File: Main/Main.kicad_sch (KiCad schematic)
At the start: 2 parts, among them J1 ATMEGA

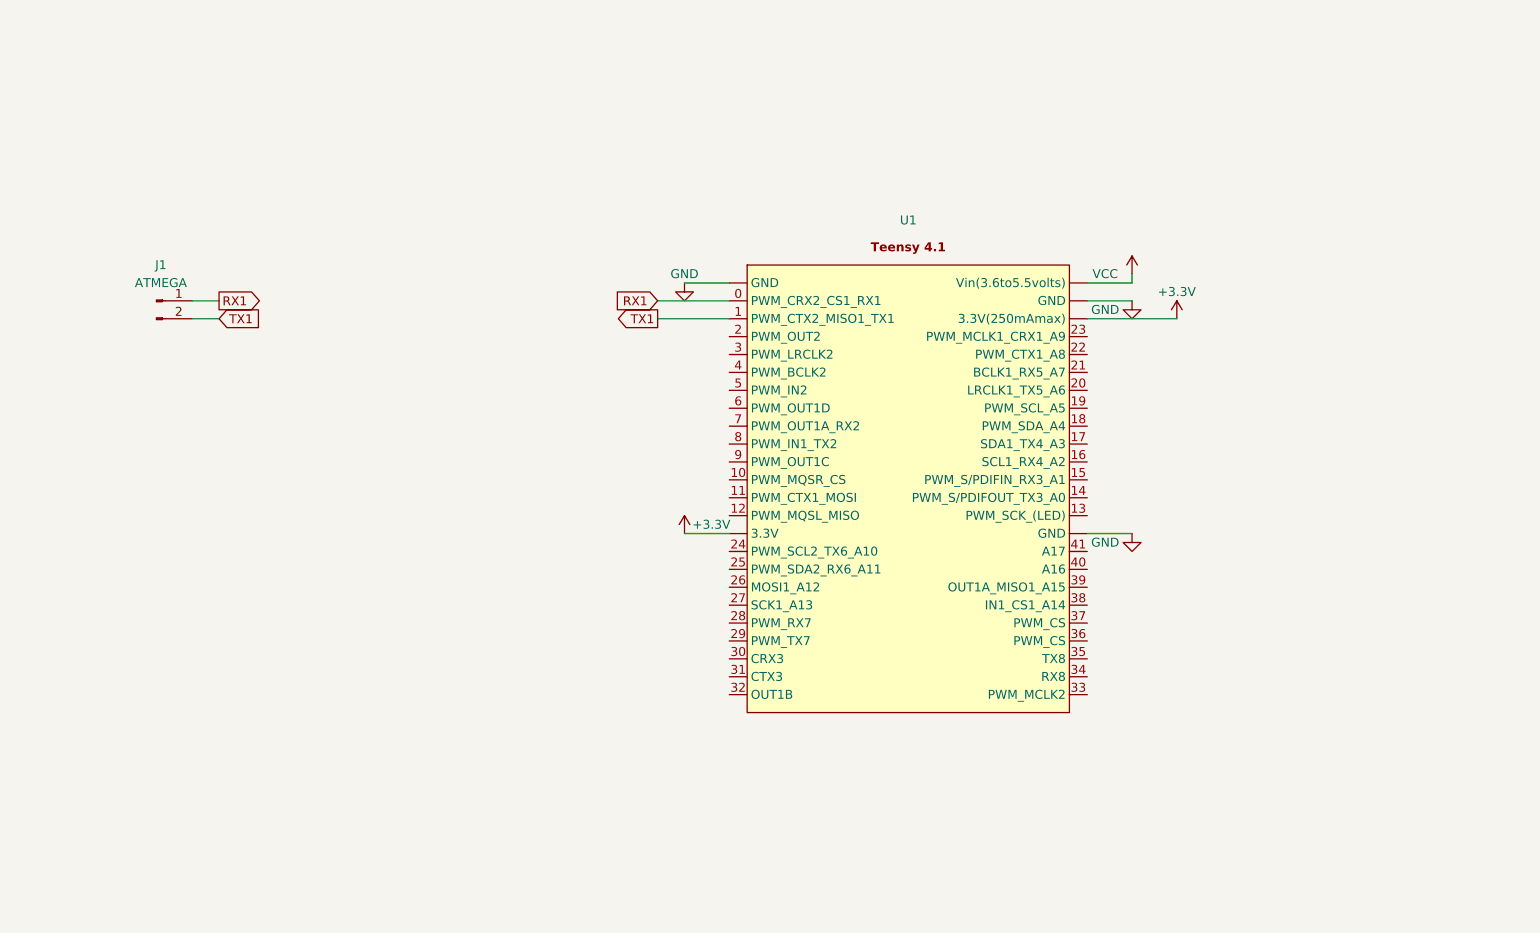
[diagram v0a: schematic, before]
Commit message: tssp58038
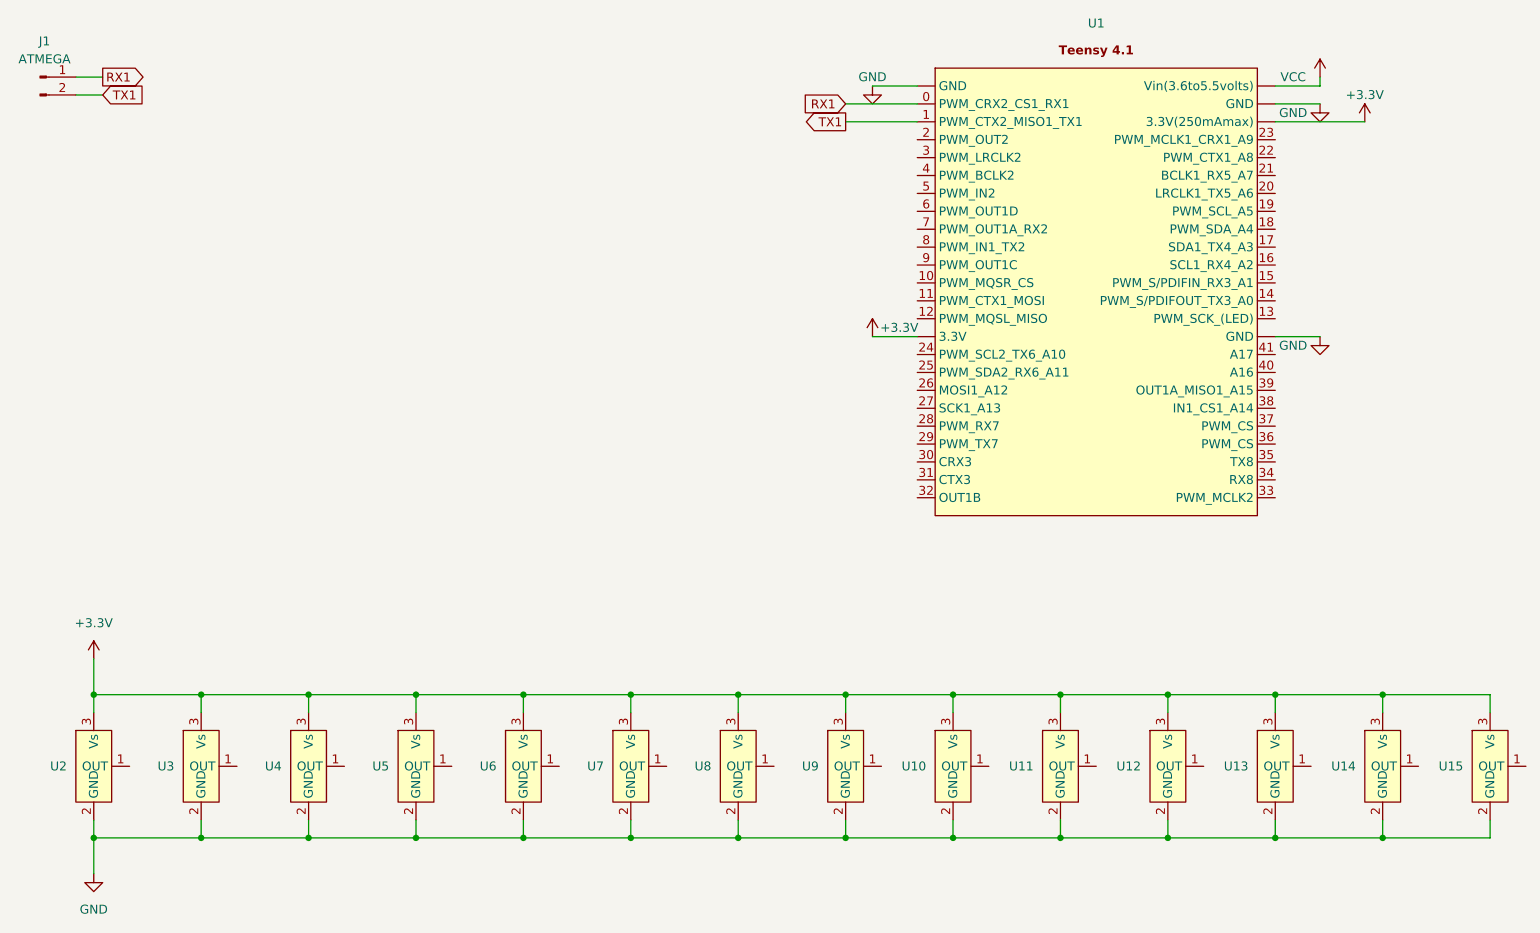
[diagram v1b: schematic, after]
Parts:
- added U10, U11, U12, U13, U14, U15, U2, U3, U4, U5, U6, U7, U8, U9: ~, symbol @admixSymbols:TSSP58038
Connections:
- net +3.3V: now also U10.3 (Vs), U11.3 (Vs), U12.3 (Vs), U13.3 (Vs), U14.3 (Vs), U15.3 (Vs), U2.3 (Vs), U3.3 (Vs), U4.3 (Vs), U5.3 (Vs), U6.3 (Vs), U7.3 (Vs), U8.3 (Vs), U9.3 (Vs)
- net GND: now also U10.2 (GND), U11.2 (GND), U12.2 (GND), U13.2 (GND), U14.2 (GND), U15.2 (GND), U2.2 (GND), U3.2 (GND), U4.2 (GND), U5.2 (GND), U6.2 (GND), U7.2 (GND), U8.2 (GND), U9.2 (GND)
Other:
- moved on the sheet: J1, U1
